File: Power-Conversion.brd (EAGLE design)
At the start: 182.9 x 114.3 mm, 46 parts, among them Q1 SUM90P10-19L, U7 LM2678

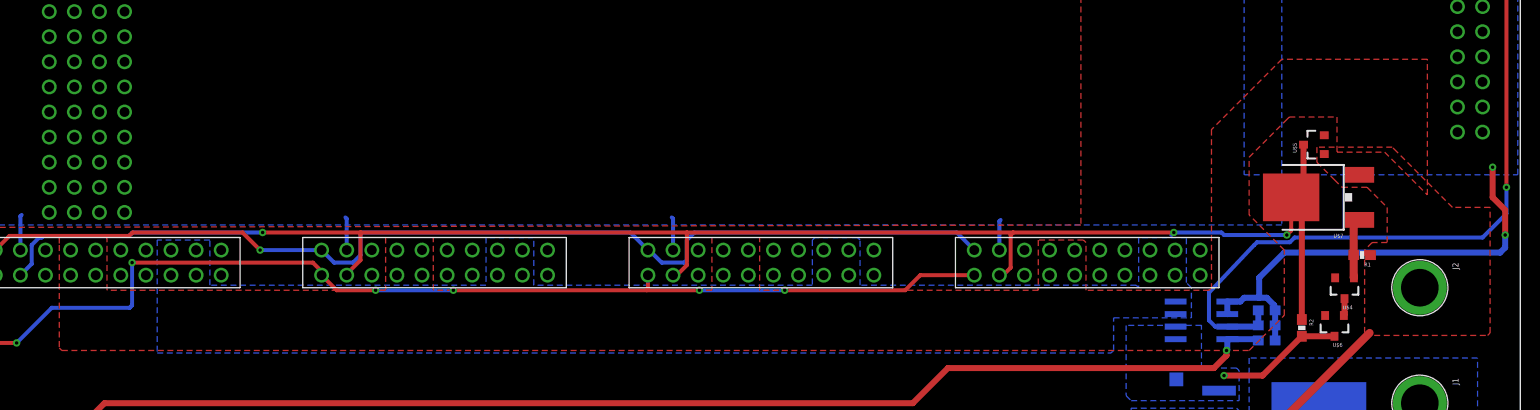
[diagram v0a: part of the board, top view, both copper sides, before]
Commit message: Stuff
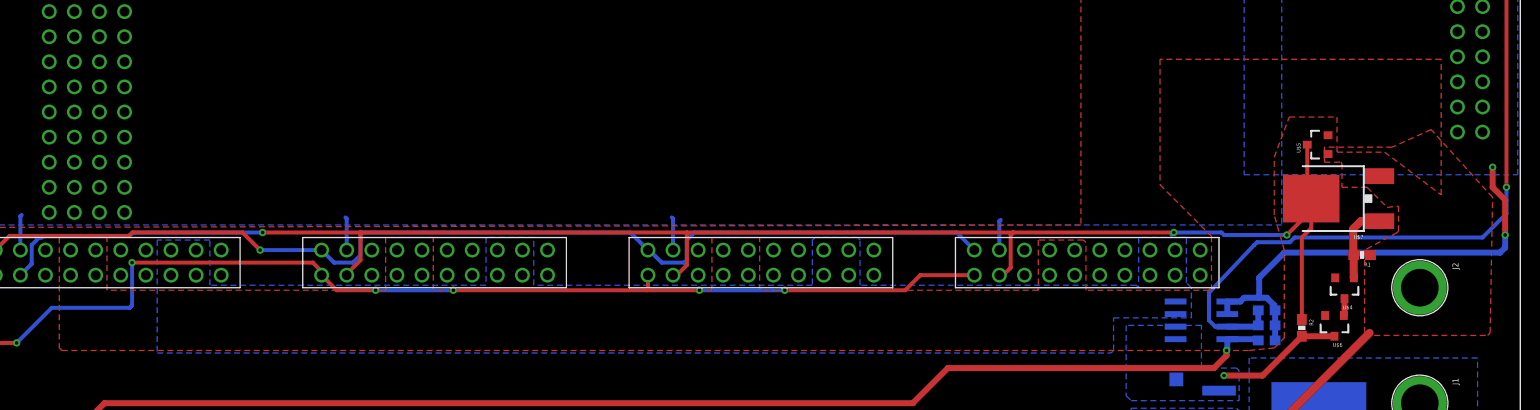
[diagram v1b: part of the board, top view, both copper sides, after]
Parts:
- moved U$7 2.04 mm to (163.3, 28.1)
- moved U$5 0.38 mm to (162.4, 33.5)
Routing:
- net ON/OFF: track 169.5 -> 173.3 mm
- net N$10: track 6.11 -> 7.96 mm
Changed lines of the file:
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@@
 <attribute name="PN-DIGI" value="BZX84C22LT1GOSCT-ND" x="165.1" y="19.05" size="1.778" layer="27" rot="R180" display="off"/>
 </element>
-<element name="U$5" library="MotherboardParts" package="SOT23-3" value="5V" x="162.052" y="33.528" rot="R90"/>
+<element name="U$5" library="MotherboardParts" package="SOT23-3" value="5V" x="162.433" y="33.528" rot="R90"/>
 <element name="U$6" library="MotherboardParts" package="SOT23-3" value="22V" x="164.084" y="15.24" rot="R180">
 <attribute name="PN-DIGI" value="BZX84C22LT1GOSCT-ND" x="164.084" y="15.24" size="1.778" layer="27" rot="R180" display="off"/>
 </element>
-<element name="U$7" library="MotherboardParts" package="DPAK" value="NMOSFET-DPAK" x="161.29" y="28.194" rot="R90">
-<attribute name="PN-DIGI" value="497-4329-1-ND" x="161.29" y="28.194" size="1.778" layer="27" rot="R90" display="off"/>
-<attribute name="VDSS" value="60V" x="161.29" y="28.194" size="1.778" layer="27" rot="R90" display="off"/>
+<element name="U$7" library="MotherboardParts" package="DPAK" value="NMOSFET-DPAK" x="163.322" y="28.067" rot="R90">
+<attribute name="PN-DIGI" value="497-4329-1-ND" x="163.322" y="28.067" size="1.778" layer="27" rot="R90" display="off"/>
+<attribute name="VDSS" value="60V" x="163.322" y="28.067" size="1.778" layer="27" rot="R90" display="off"/>
 </element>
 <element name="U$9" library="PowerComponents" package="DPAK-3" value="SWITCHMODE_SCHOTTKY" x="8.382" y="58.42" rot="MR270"/>
@@
 <wire x1="181.356" y1="23.114" x2="181.356" y2="24.384" width="0.6096" layer="16"/>
 <via x="181.356" y="24.384" extent="1-16" drill="0.35"/>
-<wire x1="181.356" y1="24.384" x2="181.356" y2="26.924" width="0.6096" layer="1"/>
-<wire x1="181.356" y1="26.924" x2="180.086" y2="28.194" width="0.6096" layer="1"/>
 <via x="180.086" y="31.242" extent="1-16" drill="0.35"/>
-<wire x1="180.086" y1="28.194" x2="180.086" y2="31.242" width="0.6096" layer="1"/>
 <polygon width="0.4064" layer="16">
 <vertex x="28.448" y="96.52"/>
@@
 <contactref element="U$8" pad="P$11"/>
 <contactref element="U$8" pad="P$10"/>
+<wire x1="181.356" y1="27.94" x2="180.086" y2="29.21" width="0.6096" layer="1"/>
+<wire x1="180.086" y1="29.21" x2="180.086" y2="31.242" width="0.6096" layer="1"/>
+<wire x1="181.356" y1="24.384" x2="181.356" y2="27.94" width="0.6096" layer="1"/>
 </signal>
 <signal name="N$9">
@@
 <contactref element="R1" pad="2"/>
 <contactref element="U$7" pad="1"/>
-<wire x1="166.6" y1="25.914" x2="166.028" y2="25.342" width="0.8128" layer="1"/>
-<wire x1="166.028" y1="25.342" x2="166.028" y2="22.352" width="0.8128" layer="1"/>
 <wire x1="166.028" y1="22.352" x2="166.028" y2="20.072" width="0.8128" layer="1"/>
 <wire x1="166.028" y1="20.072" x2="166.05" y2="20.05" width="0.8128" layer="1"/>
+<wire x1="165.989" y1="22.391" x2="166.028" y2="22.352" width="0.4064" layer="1"/>
+<wire x1="168.632" y1="25.787" x2="168.626" y2="25.781" width="0.8128" layer="1"/>
+<wire x1="168.626" y1="25.781" x2="166.751" y2="25.781" width="0.8128" layer="1"/>
+<wire x1="166.751" y1="25.781" x2="165.989" y2="25.019" width="0.8128" layer="1"/>
+<wire x1="165.989" y1="25.019" x2="165.989" y2="22.391" width="0.8128" layer="1"/>
 </signal>
 <signal name="+5V">
@@
 <vertex x="179.578" y="14.224"/>
 <vertex x="179.832" y="14.478"/>
-<vertex x="179.832" y="27.178"/>
-<vertex x="176.022" y="27.178"/>
-<vertex x="170.434" y="32.766"/>
+<vertex x="180.086" y="28.194"/>
+<vertex x="173.863" y="35.052"/>
 <vertex x="169.926" y="33.274"/>
-<vertex x="162.306" y="33.274"/>
-<vertex x="162.306" y="31.75"/>
-<vertex x="164.084" y="29.972"/>
+<vertex x="163.068" y="33.274"/>
+<vertex x="163.068" y="31.75"/>
+<vertex x="164.719" y="31.75"/>
+<vertex x="164.846" y="31.623"/>
 <vertex x="164.846" y="29.21"/>
 <vertex x="167.386" y="29.21"/>
 <vertex x="169.418" y="27.178"/>
-<vertex x="169.418" y="23.622"/>
-<vertex x="167.894" y="23.622"/>
+<vertex x="170.561" y="27.305"/>
+<vertex x="170.561" y="24.765"/>
+<vertex x="170.434" y="24.638"/>
 </polygon>
 <via x="140.462" y="4.318" extent="1-16" drill="0.35"/>
@@
 <wire x1="139.192" y1="3.302" x2="139.192" y2="2.032" width="0.8128" layer="1"/>
 <polygon width="0.4064" layer="1">
-<vertex x="35.052" y="23.368"/>
+<vertex x="35.052" y="24.13"/>
 <vertex x="35.052" y="12.954"/>
 <vertex x="35.306" y="12.7"/>
 <vertex x="155.448" y="12.7"/>
-<vertex x="156.718" y="13.97"/>
-<vertex x="159.004" y="16.256"/>
-<vertex x="159.004" y="17.526"/>
+<vertex x="157.988" y="12.954"/>
+<vertex x="159.004" y="13.97"/>
 <vertex x="159.004" y="22.86"/>
-<vertex x="155.448" y="26.416"/>
-<vertex x="155.448" y="32.258"/>
-<vertex x="159.258" y="36.068"/>
+<vertex x="157.988" y="26.416"/>
+<vertex x="157.988" y="32.258"/>
 <vertex x="159.512" y="36.322"/>
 <vertex x="164.338" y="36.322"/>
 <vertex x="164.338" y="32.766"/>
 <vertex x="169.164" y="32.766"/>
-<vertex x="173.482" y="28.448"/>
-<vertex x="173.482" y="42.164"/>
-<vertex x="158.75" y="42.164"/>
-<vertex x="151.638" y="35.052"/>
+<vertex x="174.879" y="28.448"/>
+<vertex x="174.879" y="42.164"/>
+<vertex x="146.431" y="42.164"/>
+<vertex x="146.431" y="29.464"/>
+<vertex x="151.638" y="24.257"/>
 <vertex x="151.638" y="19.05"/>
 <vertex x="151.384" y="18.796"/>
@@
 <vertex x="39.878" y="18.796"/>
 <vertex x="39.878" y="24.13"/>
-<vertex x="35.052" y="24.13"/>
 </polygon>
 <contactref element="U$20" pad="48V_GND4"/>
@@
 <contactref element="R2" pad="1"/>
 <contactref element="U$5" pad="3"/>
-<wire x1="160.952" y1="33.528" x2="160.952" y2="29.444" width="0.6096" layer="1"/>
-<wire x1="159.988" y1="28.48" x2="160.952" y2="29.444" width="0.6096" layer="1"/>
-<wire x1="159.988" y1="28.48" x2="159.702" y2="28.194" width="0.6096" layer="1"/>
-<wire x1="160.782" y1="15.836" x2="160.782" y2="27.686" width="0.6096" layer="1"/>
+<wire x1="160.952" y1="29.444" x2="159.988" y2="28.48" width="0.6096" layer="1"/>
+<wire x1="159.988" y1="28.48" x2="161.734" y2="28.067" width="0.6096" layer="1"/>
 <wire x1="160.782" y1="27.686" x2="159.988" y2="28.48" width="0.6096" layer="1"/>
-<wire x1="159.702" y1="28.194" x2="159.702" y2="24.828" width="0.4064" layer="1"/>
-<wire x1="159.702" y1="24.828" x2="159.258" y2="24.384" width="0.4064" layer="1"/>
 <via x="159.258" y="24.384" extent="1-16" drill="0.35"/>
 <wire x1="159.258" y1="24.384" x2="152.908" y2="24.384" width="0.4064" layer="16"/>
@@
 <wire x1="33.4344" y1="24.2904" x2="42.1156125" y2="24.2904" width="0.4064" layer="16"/>
 <wire x1="42.4632125" y1="24.638" x2="55.626" y2="24.638" width="0.4064" layer="16"/>
+<wire x1="159.702" y1="26.606" x2="160.782" y2="27.686" width="0.4064" layer="1"/>
+<wire x1="160.782" y1="25.908" x2="160.782" y2="27.686" width="0.4064" layer="1"/>
+<wire x1="159.258" y1="24.384" x2="160.782" y2="25.908" width="0.4064" layer="1"/>
+<wire x1="160.782" y1="15.836" x2="160.782" y2="24.13" width="0.4064" layer="1"/>
+<wire x1="161.734" y1="25.082" x2="161.734" y2="28.067" width="0.4064" layer="1"/>
+<wire x1="160.782" y1="24.13" x2="161.734" y2="25.082" width="0.4064" layer="1"/>
+<wire x1="161.333" y1="33.528" x2="161.333" y2="29.825" width="0.4064" layer="1"/>
+<wire x1="161.333" y1="29.825" x2="160.952" y2="29.444" width="0.4064" layer="1"/>
 </signal>
 <signal name="+12V_1">
